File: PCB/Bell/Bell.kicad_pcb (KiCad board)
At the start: 2 copper layers, 38.3 x 28.7 mm, 31 parts, among them J1 USB-C, J2 POWER, J3 Conn_01x08, J5 Conn_01x05, J6 Conn_01x02, J7 Shelly, U1 MD8942, U3 ISL89410, U4 ISL89410, U6 ESP32-S3-MINI-1, U7 AA, U8 QR

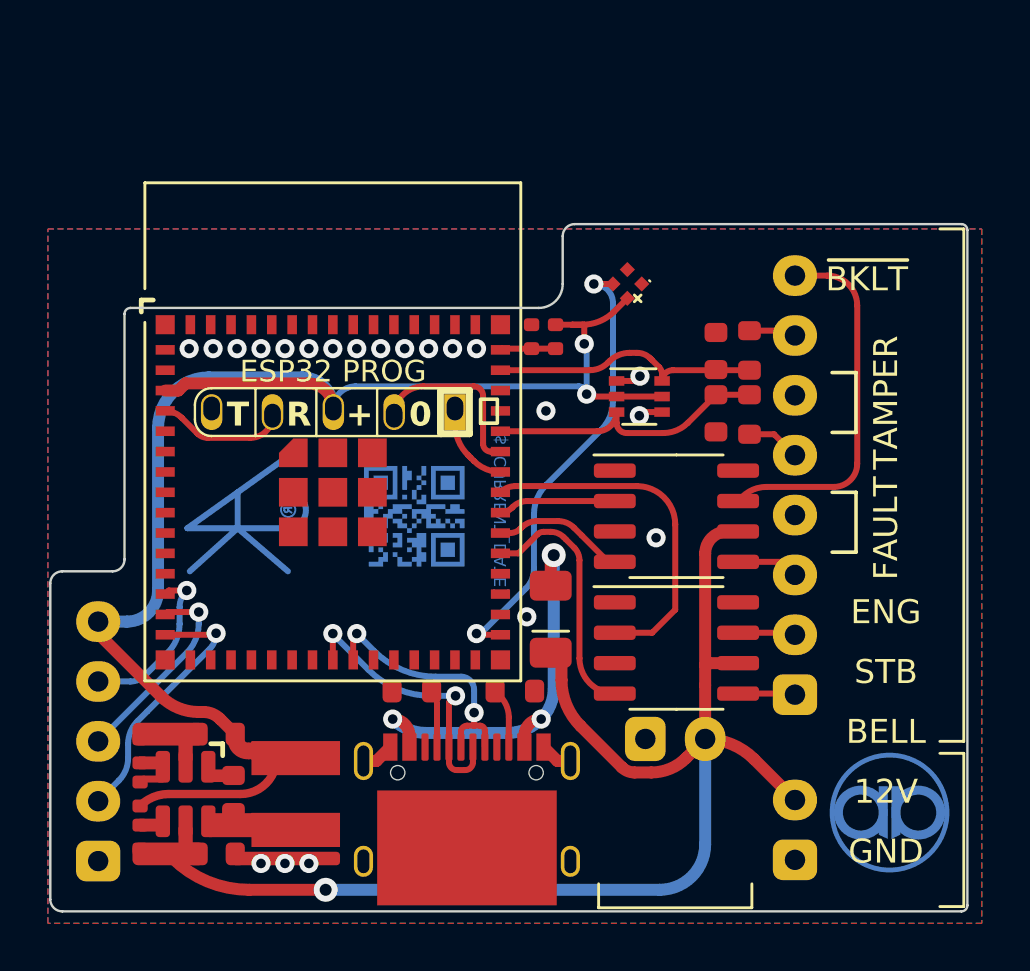
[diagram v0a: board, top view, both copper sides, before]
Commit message: Clean up a lot
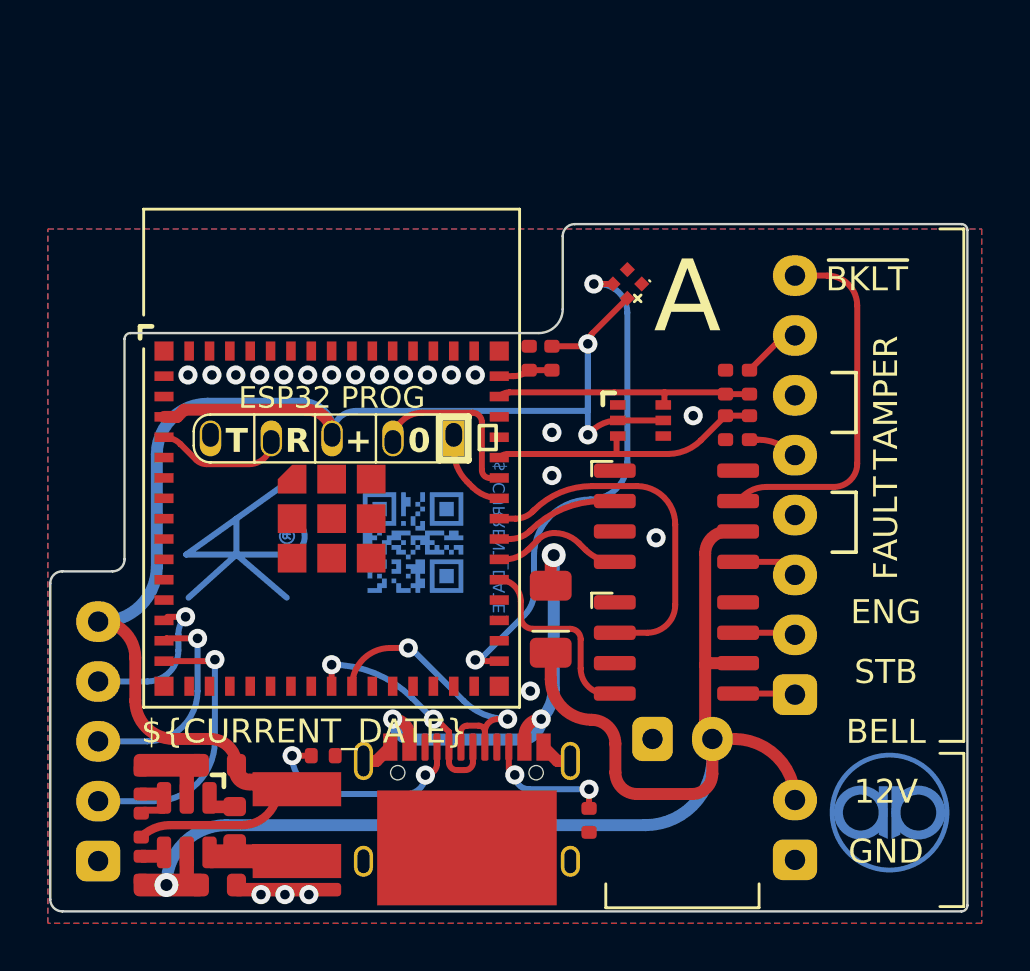
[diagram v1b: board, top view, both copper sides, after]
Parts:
- C2, C3: footprint RevK:C_0603 -> RevK:C_0402
- D1: footprint Package_TO_SOT_SMD:SOT-363_SC-70-6 -> RevK:SOT-363_SC-70-6
- R4, R5, R6, R7: footprint RevK:R_0603 -> RevK:R_0402
- U3, U4: footprint Package_SO:SO-8_3.9x4.9mm_P1.27mm -> RevK:SO-8_3.9x4.9mm_P1.27mm
- moved L2 22.0 mm to (80.4, 56.9), turned to 90 degrees
- moved C9 18.8 mm to (77.8, 56.9), turned to 90 degrees
- moved C7 18.5 mm to (77.1, 54.4), turned to 180 degrees
- moved C1 15.5 mm to (77.1, 59.4), turned to 180 degrees
- moved R2 13.6 mm to (73.9, 55.1), turned to 90 degrees
- moved R3 12.3 mm to (73.9, 58.7), turned to 90 degrees
- moved R1 11.1 mm to (73.9, 56.9), turned to 90 degrees
- moved R6 6.23 mm to (92.6, 56.7), turned to 90 degrees
- moved R5 4.58 mm to (81.5, 54.0), turned to 0 degrees
- moved C2 1.36 mm to (98.3, 38.4)
- moved R4 1.32 mm to (99.3, 38.4)
- moved U1 1.30 mm to (75.8, 56.9)
- moved U6 1.10 mm to (81.8, 44.1)
- moved AJK1 1.10 mm to (77.9, 45.6)
- moved J7 1.10 mm to (81.9, 40.8)
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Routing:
- net Net-(J1-CC1): track 2.40 -> 9.06 mm, vias 0 -> 2
- net +3V3: track 55.9 -> 60.2 mm
- net Net-(J1-CC2): track 2.52 -> 5.51 mm, vias 0 -> 2
- net LED: track 19.1 -> 21.5 mm
- net OUT1: track 10.6 -> 8.23 mm
- net GND: track 4.79 -> 2.72 mm
- net D-: track 12.0 -> 9.98 mm
- net +12V: track 53.8 -> 55.2 mm
- net D+: track 11.0 -> 12.2 mm
- net T: track 1.98 -> 2.73 mm
- net GPSRX: track 11.0 -> 11.8 mm
- net GPSTICK: track 7.12 -> 6.48 mm
- net VBUS: track 17.9 -> 18.5 mm
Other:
- outline, holes or cut-outs redrawn
- board text added: "${CURRENT_DATE}"
- board text added: "+"
- board text added: "A"
- board text added: "⏚"

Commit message: LEDs
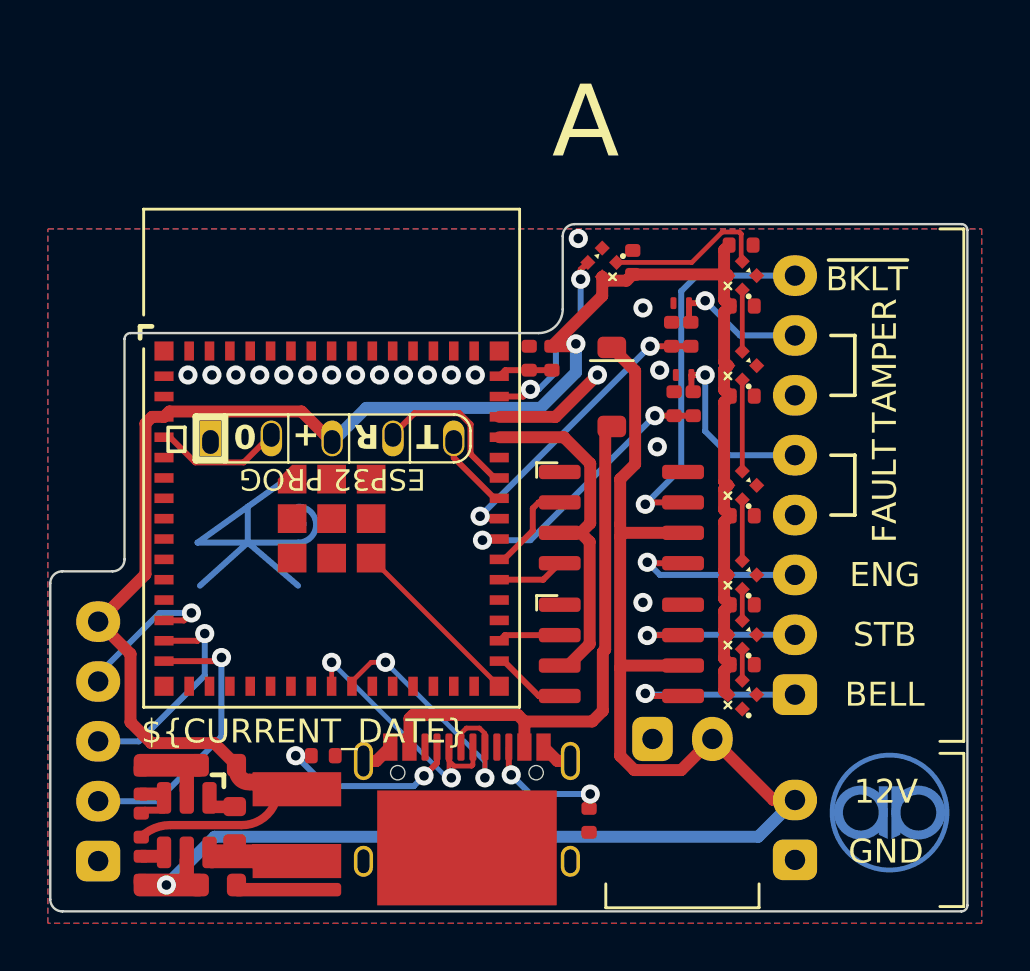
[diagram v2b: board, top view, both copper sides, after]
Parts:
- removed U8: QR, RevK:QR-SS
- added C10: 100nF, RevK:C_0402, F.Cu at (99.0, 39.0)
- added C11: 100nF, RevK:C_0402, F.Cu at (99.0, 44.0)
- added C12: 100nF, RevK:C_0402, F.Cu at (99.0, 47.7)
- added C13: 100nF, RevK:C_0402, F.Cu at (99.0, 50.2)
- added C4: 100nF, RevK:C_0402, F.Cu at (94.4, 33.4)
- added C5: 100nF, RevK:C_0402, F.Cu at (99.0, 32.7)
- added C6: 100nF, RevK:C_0402, F.Cu at (99.0, 35.2)
- added D10: ~, RevK:DFN1006-2L, F.Cu at (96.5, 38.1)
- added D2: XL-1010RGBC-WS2812B, RevK:SMD1010, F.Cu at (99.0, 34.0)
- added D4: XL-1010RGBC-WS2812B, RevK:SMD1010, F.Cu at (99.0, 37.7)
- added D6: XL-1010RGBC-WS2812B, RevK:SMD1010, F.Cu at (99.0, 42.7)
- added D7: XL-1010RGBC-WS2812B, RevK:SMD1010, F.Cu at (99.0, 46.5)
- added D8: XL-1010RGBC-WS2812B, RevK:SMD1010, F.Cu at (99.0, 49.0)
- added D9: XL-1010RGBC-WS2812B, RevK:SMD1010, F.Cu at (99.0, 51.5)
- D1: value BAV99S -> ~; footprint RevK:SOT-363_SC-70-6 -> RevK:DFN1006-2L
- D3: value D -> MBR0530; footprint RevK:D_1206 -> RevK:D_SOD-123
- J1: value USB-C -> USB-C-Socket-V; footprint RevK:USC16-TR -> RevK:USB-C-Socket-H
- moved D3 10.0 mm to (93.5, 38.6), turned to -90 degrees
- moved D1 5.19 mm to (96.5, 35.1), turned to 180 degrees
- moved R4 3.16 mm to (96.8, 36.4)
- moved C2 3.01 mm to (96.0, 36.4)
- moved R7 2.55 mm to (97.0, 39.3), turned to -90 degrees
- moved C3 2.37 mm to (96.2, 39.3), turned to 90 degrees
- moved U3 2.30 mm to (94.0, 49.6)
- moved U4 2.30 mm to (94.0, 44.1)
- moved D5 1.38 mm to (93.2, 33.4)
- moved AJK1 0.69 mm to (78.3, 45.1)
- turned J7 to 180 degrees
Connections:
- D1 pad 1: GND -> T
- D1 pad 2: +3V3 -> GND
- D5 pad 1: unconnected-(D5-O-Pad1) -> Net-(D2-I)
- D5 pad 2: +3V3 -> +3.3V
- D5 pad 4: LED -> RGB
- J5 pad 5: +3V3 -> +3.3V
- J7 pad 1: Net-(J7-GND) -> GND
- J7 pad 3: +3V3 -> +3.3V
- J7 pad 5: GND -> Net-(J7-Tx)
- R8 pad 1: +3V3 -> +3.3V
- U1 pad 8: +3V3 -> +3.3V
- U6 pad 3: +3V3 -> +3.3V
- U6 pad 31: LED -> OUT1
- U6 pad 32: unconnected-(U6-GPIO36-Pad32) -> OUT2
- U6 pad 35: OUT1 -> OUT3
- U6 pad 36: OUT3 -> OUT4
- U6 pad 37: OUT4 -> IN2
- U6 pad 38: OUT2 -> IN1
- U6 pad 39: Net-(J7-GND) -> Net-(J7-Tx)
- U6 pad 4: Net-(J7-Rx) -> Net-(J7-0)
- U6 pad 40: Net-(J7-0) -> Net-(J7-Rx)
- U6 pad 41: IN2 -> unconnected-(U6-GPIO45-Pad41)
- U6 pad 44: IN1 -> RGB
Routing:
- net +3.3V: track 0.00 -> 71.1 mm, vias 0 -> 1
- net +3V3: track 60.2 -> 0.00 mm, vias 2 -> 0
- net GND: track 2.72 -> 29.7 mm, vias 21 -> 19
- net LED: track 21.5 -> 0.00 mm, vias 2 -> 0
- net OUT2: track 15.1 -> 2.62 mm
- net RGB: track 0.00 -> 7.92 mm, vias 0 -> 2
- net Net-(D2-I): track 0.00 -> 6.92 mm
- net FAULT: track 2.06 -> 7.82 mm, vias 0 -> 1
- net BELL: track 2.39 -> 7.89 mm, vias 0 -> 1
- net ENGHOLD: track 2.60 -> 7.90 mm, vias 0 -> 1
- net STB: track 2.41 -> 7.68 mm, vias 0 -> 1
- net OUT1: track 8.23 -> 3.13 mm
- net +12V: track 55.2 -> 60.1 mm
- net VBUS: track 18.5 -> 22.7 mm, vias 3 -> 0
- net Net-(D4-O): track 0.00 -> 3.80 mm
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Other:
- board text added: "35"
- board text added: "36"
- board text added: "RGB:46"
- board text removed: "45"
- board text removed: "46"
- board text removed: "RGB:33"
